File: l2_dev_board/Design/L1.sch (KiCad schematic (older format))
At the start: 13 parts, among them U502 XS1-L1-128

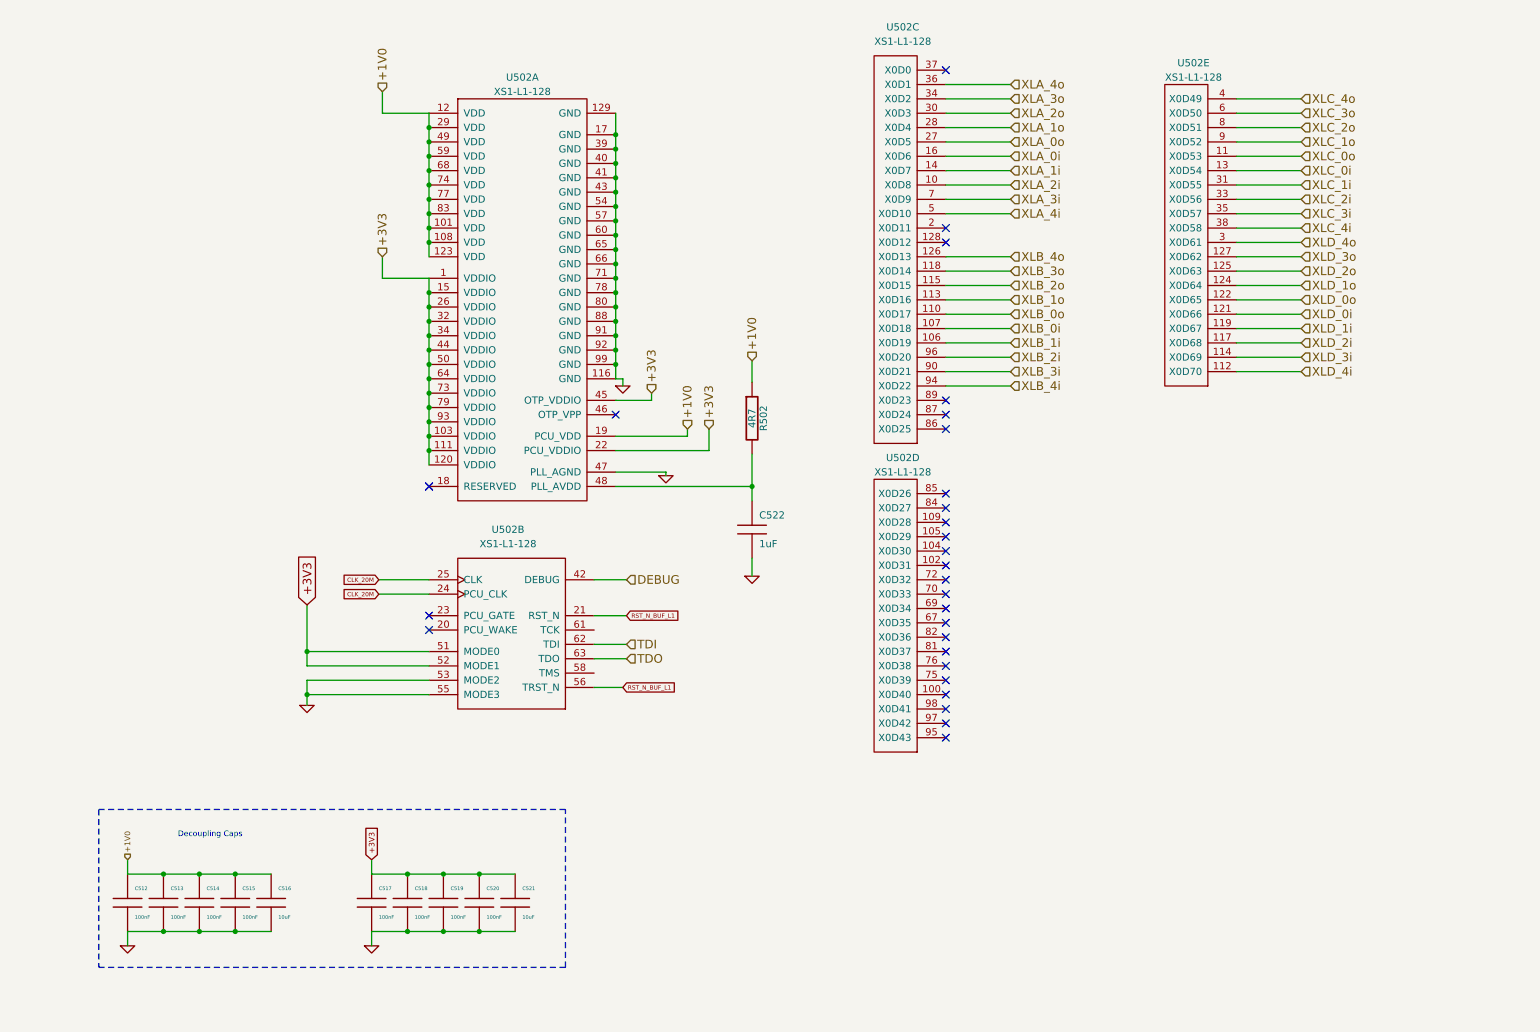
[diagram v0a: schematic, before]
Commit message: Isolated L1 stuff (inc. JTAG) in single sheet. Added buffered for the L2's JTAG control signals.
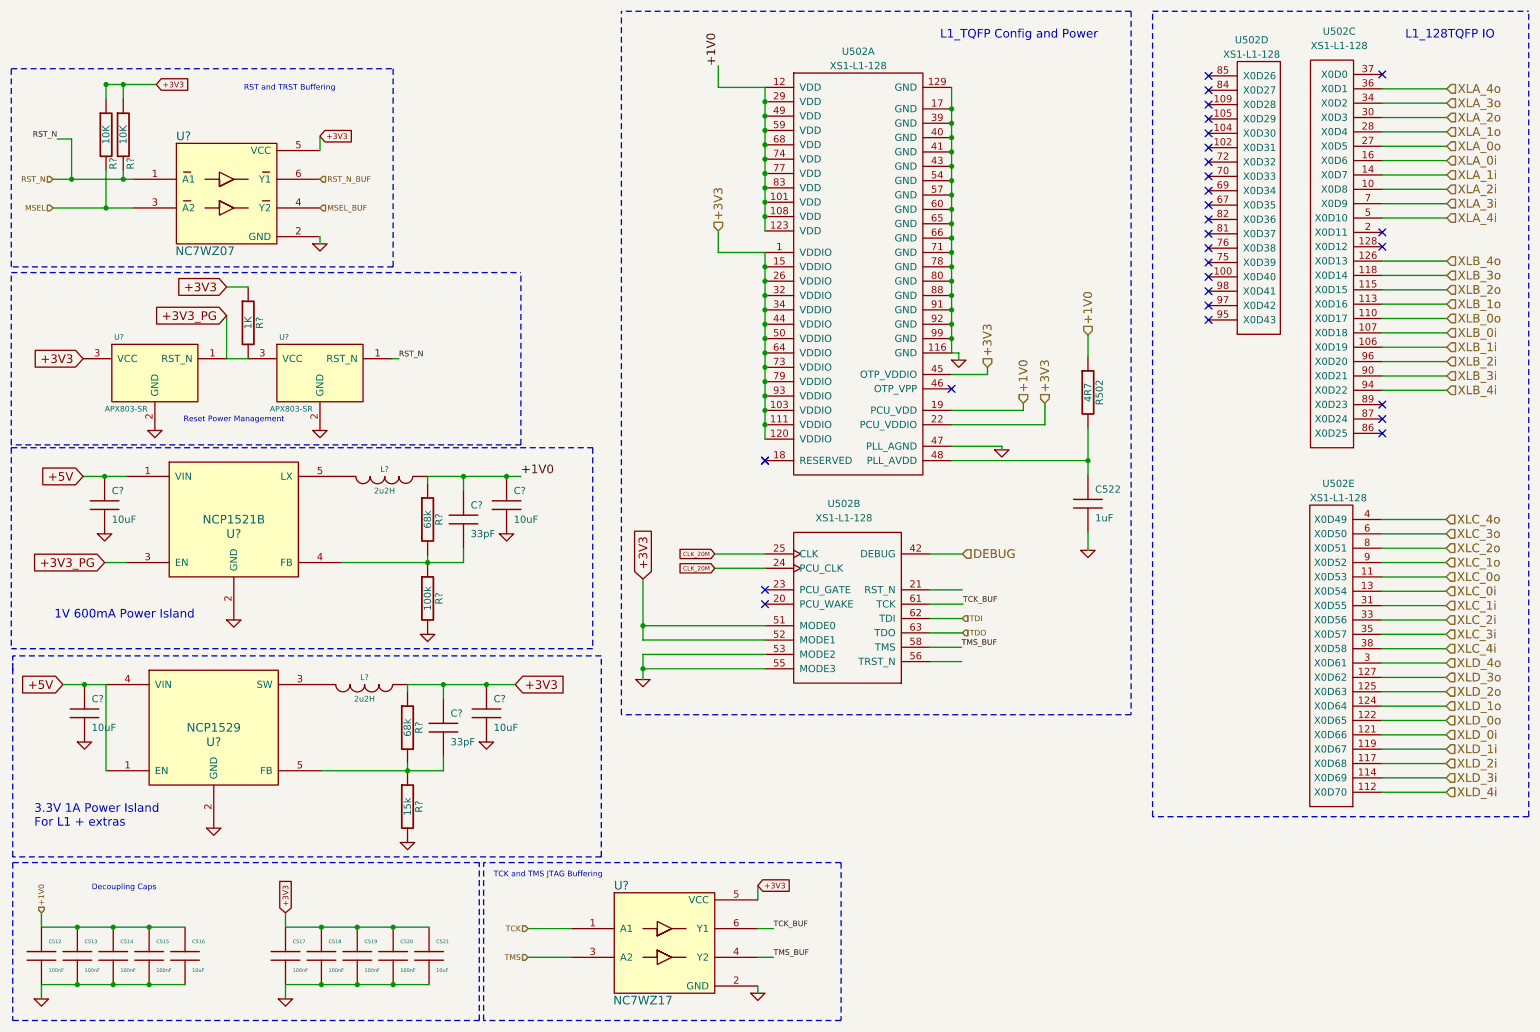
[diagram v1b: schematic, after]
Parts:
- added C? (x4): 10uF, symbol C
- added C? (x2): 33pF, symbol C
- added L? (x2): 2u2H, symbol INDUCTOR
- added R? (x2): 10K, symbol R
- added R?: 1K, symbol R
- added R? (x2): 68k, symbol R
- added R?: 15k, symbol R
- added R?: 100k, symbol R
- added U?: NC7WZ17, symbol NC7WZ17
- added U?: NC7WZ07, symbol NC7WZ07
- added U? (x2): APX803-SR, SOT23R, symbol APX803-SR
- added U?: NCP1529, symbol NCP1529
- added U?: NCP1521B, symbol NCP1521B
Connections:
- net +1V0: now also C?.1, C?.1, L?.1, R?.1
- net +3V3: now also C?.1, C?.1, L?.1, R?.1, R?.1, R?.1, R?.1, U?.3 (VCC), U?.5 (VCC), U?.5 (VCC)
- net GND: now also C?.2, C?.2, C?.2, C?.2, R?.2, R?.2, U?.2 (GND), U?.2 (GND), U?.2 (GND), U?.2 (GND), U?.2 (GND), U?.2 (GND)
- net TMS_BUF: now reaches U502.58 (TMS)
- net TMS_BUF: now also U?.4 (Y2)
- net TCK_BUF: now reaches U502.61 (TCK)
- net TCK_BUF: now also U?.6 (Y1)
- net RST_N_BUF_L1: no longer names the net of U502.21 (RST_N)
- net RST_N_BUF_L1: no longer U502.56 (TRST_N)
- new net: L?.2, U?.3 (SW)
- new net: C?.2, R?.1, R?.2, U?.5 (FB)
- new net: L?.2, U?.5 (LX)
- new net: C?.2, R?.1, R?.2, U?.4 (FB)
- new net +3V3_PG: R?.2, U?.1 (RST_N), U?.3 (EN), U?.3 (VCC)
- new net +5V: C?.1, C?.1, U?.1 (EN), U?.1 (VIN), U?.4 (VIN)
- new net MSEL: R?.2, U?.3 (A2)
- new net MSEL_BUF: U?.4 (Y2)
- new net RST_N: R?.2, U?.1 (A1), U?.1 (RST_N)
- new net RST_N_BUF: U?.6 (Y1)
- new net TCK: U?.1 (A1)
- new net TMS: U?.3 (A2)
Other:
- note added: "1V 600mA Power Island"
- note added: "3.3V 1A Power Island\nFor L1 + extras"
- note added: "L1_128TQFP IO"
- note added: "L1_TQFP Config and Power"
- note added: "RST and TRST Buffering"
- note added: "Reset Power Management"
- note added: "TCK and TMS JTAG Buffering"
- moved on the sheet: C512, C513, C514, C515, C516, C517, C518, C519, C520, C521, C522, R502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

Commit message: removing old buffering and wanted to check point
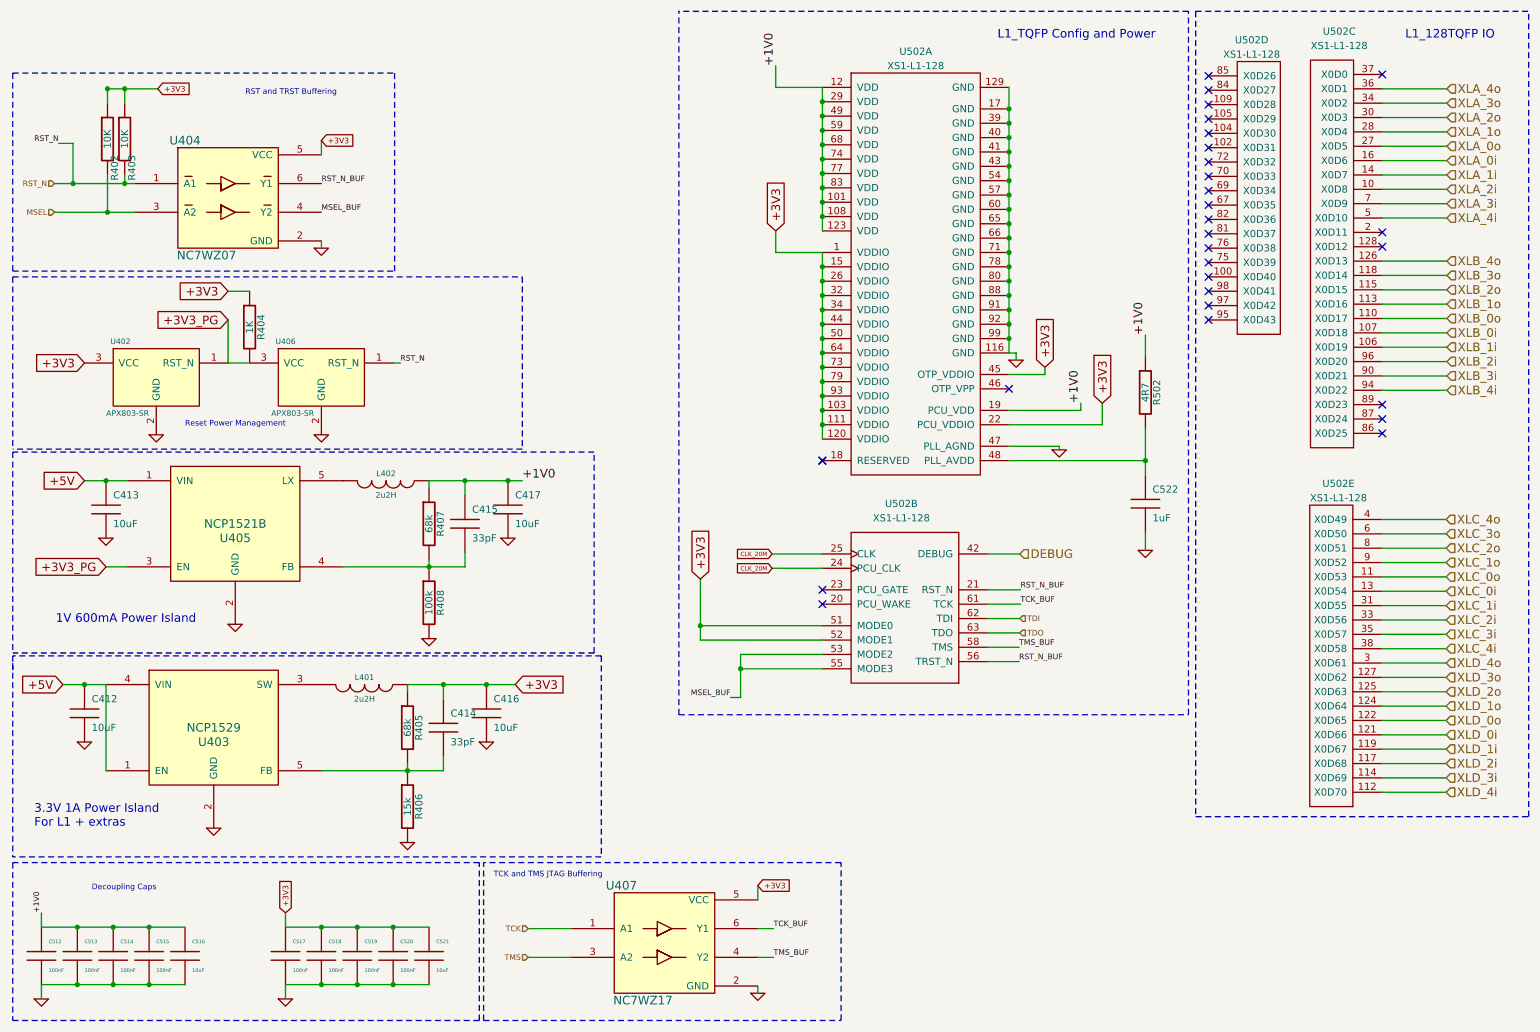
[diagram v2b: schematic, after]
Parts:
- gave numbers to parts that had none: 21
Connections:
- net GND: no longer U502.53 (MODE2), U502.55 (MODE3)
- net MSEL_BUF: now also U502.53 (MODE2), U502.55 (MODE3)
- net RST_N_BUF: now also U502.21 (RST_N), U502.56 (TRST_N)
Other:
- moved on the sheet: C413, C415, C417, C522, L402, R402, R403, R404, R407, R408, R502, U402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

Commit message: missing header connector for 2 L2s. Find space!
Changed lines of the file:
@@
-EESchema Schematic File Version 2  date 28/07/2011 17:12:08
+EESchema Schematic File Version 2  date 28/07/2011 17:28:18
 LIBS:power
 LIBS:device
@@
 Comment4 ""
 $EndDescr
-Text Label 800  6920 1    39   ~ 0
-+1V0
-Wire Wire Line
-	5670 5420 5600 5420
+Wire Wire Line
+	5600 5420 5670 5420
 Wire Wire Line
 	5670 5420 5670 5120
@@
 	3850 7670 3850 6570
 Wire Wire Line
-	800  7420 800  7520
-Wire Wire Line
-	2500 7420 2500 7520
+	800  7520 800  7420
+Wire Wire Line
+	2500 7520 2500 7420
 Connection ~ 3000 7420
 Connection ~ 3000 7020
@@
 Connection ~ 1300 7020
 Wire Wire Line
-	800  7020 800  6920
+	800  6920 800  7020
 Connection ~ 1050 7020
 Wire Wire Line
-	1800 7020 800  7020
+	800  7020 1800 7020
 Connection ~ 1550 7020
 Connection ~ 1550 7420
 Wire Wire Line
-	1800 7420 800  7420
+	800  7420 1800 7420
 Connection ~ 1050 7420
 Wire Wire Line
-	2500 7020 2500 6920
+	2500 6920 2500 7020
 Connection ~ 2750 7020
 Wire Wire Line
-	3500 7020 2500 7020
+	2500 7020 3500 7020
 Connection ~ 3250 7020
 Connection ~ 3250 7420
 Wire Wire Line
-	3500 7420 2500 7420
+	2500 7420 3500 7420
 Connection ~ 2750 7420
 Wire Notes Line
@@
 	2750 2290 2750 2240
 Wire Wire Line
-	1260 1180 1260 1280
+	1260 1280 1260 1180
 Connection ~ 1260 1180
 Wire Wire Line
@@
 Connection ~ 1380 1840
 Wire Wire Line
-	1610 1180 1260 1180
+	1260 1180 1610 1180
 Wire Notes Line
 	4700 5130 600  5130
 Wire Wire Line
-	1250 5330 1250 5930
-Wire Wire Line
-	3600 5930 3600 5830
+	1250 5930 1250 5330
+Wire Wire Line
+	3600 5830 3600 5930
 Connection ~ 3900 5330
 Wire Wire Line
@@
 	3350 5330 3350 5380
 Wire Wire Line
-	950  5330 1250 5330
+	1250 5330 950  5330
 Connection ~ 1100 5330
 Wire Wire Line
-	2750 5930 3600 5930
+	3600 5930 2750 5930
 Connection ~ 3350 5930
 Wire Wire Line
@@
 	4650 5110 600  5110
 Wire Wire Line
-	3750 4510 3750 4410
+	3750 4410 3750 4510
 Connection ~ 4050 3910
 Wire Wire Line
@@
 Connection ~ 1250 3910
 Wire Wire Line
-	2900 4510 3750 4510
+	3750 4510 2900 4510
 Connection ~ 3500 4510
 Wire Wire Line
@@
 Wire Wire Line
 	7620 4670 7390 4670
+Text Label 800  6920 1    39   ~ 0
++1V0
 Text GLabel 7790 3120 1    60   Input ~ 0
 +3V3
@@
 1V 600mA Power Island
 $Comp
-L GND #PWR036
+L GND #PWR031
 U 1 1 4E3166D5
 P 4050 4310
-F 0 "#PWR036" H 4050 4310 30  0001 C CNN
+F 0 "#PWR031" H 4050 4310 30  0001 C CNN
 F 1 "GND" H 4050 4240 30  0001 C CNN
 	1    4050 4310
@@
 $EndComp
 $Comp
-L GND #PWR037
+L GND #PWR032
 U 1 1 4E3166D4
 P 3500 5010
-F 0 "#PWR037" H 3500 5010 30  0001 C CNN
+F 0 "#PWR032" H 3500 5010 30  0001 C CNN
 F 1 "GND" H 3500 4940 30  0001 C CNN
 	1    3500 5010
@@
 $EndComp
 $Comp
-L GND #PWR038
+L GND #PWR033
 U 1 1 4E3166CE
 P 2150 4910
-F 0 "#PWR038" H 2150 4910 30  0001 C CNN
+F 0 "#PWR033" H 2150 4910 30  0001 C CNN
 F 1 "GND" H 2150 4840 30  0001 C CNN
 	1    2150 4910
@@
 $EndComp
 $Comp
-L GND #PWR039
+L GND #PWR034
 U 1 1 4E3166CD
 P 1250 4310
-F 0 "#PWR039" H 1250 4310 30  0001 C CNN
+F 0 "#PWR034" H 1250 4310 30  0001 C CNN
 F 1 "GND" H 1250 4240 30  0001 C CNN
 	1    1250 4310
@@
 3.3V 1A Power Island\nFor L1 + extras
 $Comp
-L GND #PWR040
+L GND #PWR035
 U 1 1 4E316650
 P 3900 5730
-F 0 "#PWR040" H 3900 5730 30  0001 C CNN
+F 0 "#PWR035" H 3900 5730 30  0001 C CNN
 F 1 "GND" H 3900 5660 30  0001 C CNN
 	1    3900 5730
@@
 $EndComp
 $Comp
-L GND #PWR041
+L GND #PWR036
 U 1 1 4E31664F
 P 3350 6430
-F 0 "#PWR041" H 3350 6430 30  0001 C CNN
+F 0 "#PWR036" H 3350 6430 30  0001 C CNN
 F 1 "GND" H 3350 6360 30  0001 C CNN
 	1    3350 6430
@@
 $EndComp
 $Comp
-L GND #PWR042
+L GND #PWR037
 U 1 1 4E316649
 P 2000 6330
-F 0 "#PWR042" H 2000 6330 30  0001 C CNN
+F 0 "#PWR037" H 2000 6330 30  0001 C CNN
 F 1 "GND" H 2000 6260 30  0001 C CNN
 	1    2000 6330
@@
 $EndComp
 $Comp
-L GND #PWR043
+L GND #PWR038
 U 1 1 4E316648
 P 1100 5730
-F 0 "#PWR043" H 1100 5730 30  0001 C CNN
+F 0 "#PWR038" H 1100 5730 30  0001 C CNN
 F 1 "GND" H 1100 5660 30  0001 C CNN
 	1    1100 5730
@@
 +3V3_PG
 $Comp
-L GND #PWR044
+L GND #PWR039
 U 1 1 4E316549
 P 2750 3590
-F 0 "#PWR044" H 2750 3590 30  0001 C CNN
+F 0 "#PWR039" H 2750 3590 30  0001 C CNN
 F 1 "GND" H 2750 3520 30  0001 C CNN
 	1    2750 3590
@@
 $EndComp
 $Comp
-L GND #PWR045
+L GND #PWR040
 U 1 1 4E316548
 P 1600 3590
-F 0 "#PWR045" H 1600 3590 30  0001 C CNN
+F 0 "#PWR040" H 1600 3590 30  0001 C CNN
 F 1 "GND" H 1600 3520 30  0001 C CNN
 	1    1600 3590
@@
 +3V3
 $Comp
-L GND #PWR046
+L GND #PWR041
 U 1 1 4E31647C
 P 2750 2290
-F 0 "#PWR046" H 2750 2290 30  0001 C CNN
+F 0 "#PWR041" H 2750 2290 30  0001 C CNN
 F 1 "GND" H 2750 2220 30  0001 C CNN
 	1    2750 2290
@@
 +3V3
 $Comp
-L GND #PWR047
+L GND #PWR042
 U 1 1 4E31626A
 P 5790 7480
-F 0 "#PWR047" H 5790 7480 30  0001 C CNN
+F 0 "#PWR042" H 5790 7480 30  0001 C CNN
 F 1 "GND" H 5790 7410 30  0001 C CNN
 	1    5790 7480
@@
 $EndComp
 $Comp
-L GND #PWR048
+L GND #PWR043
 U 1 1 4E3024EA
 P 800 7520
-F 0 "#PWR048" H 800 7520 30  0001 C CNN
+F 0 "#PWR043" H 800 7520 30  0001 C CNN
 F 1 "GND" H 800 7450 30  0001 C CNN
 	1    800  7520
@@
 +3V3
 $Comp
-L GND #PWR049
+L GND #PWR044
 U 1 1 4E3024E9
 P 2500 7520
-F 0 "#PWR049" H 2500 7520 30  0001 C CNN
+F 0 "#PWR044" H 2500 7520 30  0001 C CNN
 F 1 "GND" H 2500 7450 30  0001 C CNN
 	1    2500 7520
@@
 NoConn ~ 6240 4670
 $Comp
-L GND #PWR050
+L GND #PWR045
 U 1 1 4E301046
 P 7890 3695
-F 0 "#PWR050" H 7890 3695 30  0001 C CNN
+F 0 "#PWR045" H 7890 3695 30  0001 C CNN
 F 1 "GND" H 7890 3625 30  0001 C CNN
 	1    7890 3695
@@
 $EndComp
 $Comp
-L GND #PWR051
+L GND #PWR046
 U 1 1 4E301022
 P 8490 4395
-F 0 "#PWR051" H 8490 4395 30  0001 C CNN
+F 0 "#PWR046" H 8490 4395 30  0001 C CNN
 F 1 "GND" H 8490 4325 30  0001 C CNN
 	1    8490 4395
@@
 NoConn ~ 6240 3770
 $Comp
-L GND #PWR052
+L GND #PWR047
 U 1 1 4E300DCB
 P 7590 3070
-F 0 "#PWR052" H 7590 3070 30  0001 C CNN
+F 0 "#PWR047" H 7590 3070 30  0001 C CNN
 F 1 "GND" H 7590 3000 30  0001 C CNN
 	1    7590 3070
